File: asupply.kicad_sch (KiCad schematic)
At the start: 98 parts, among them U10 LT3081xDF, U11 LT3042xMSE, U12 LT3045xMSE, U13 LT3045xMSE, U14 LT3042xMSE, U15 LT3094xMSE, U16 LT3042xMSE, U9 LTC3261

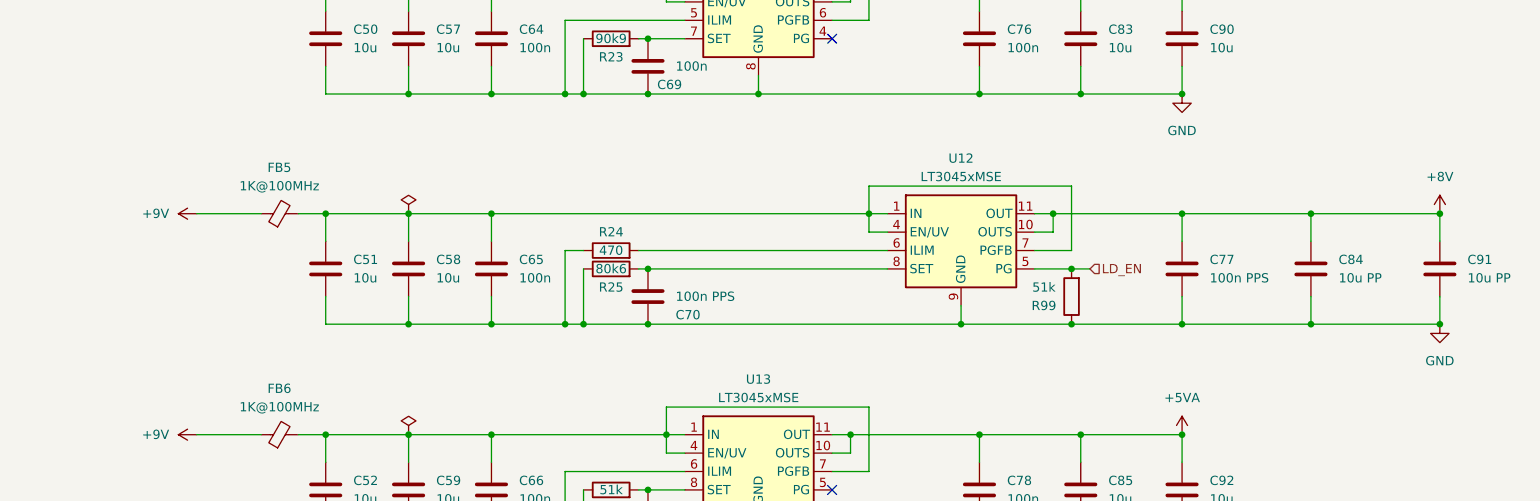
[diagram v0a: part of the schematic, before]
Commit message: sch: Fix Issue #14
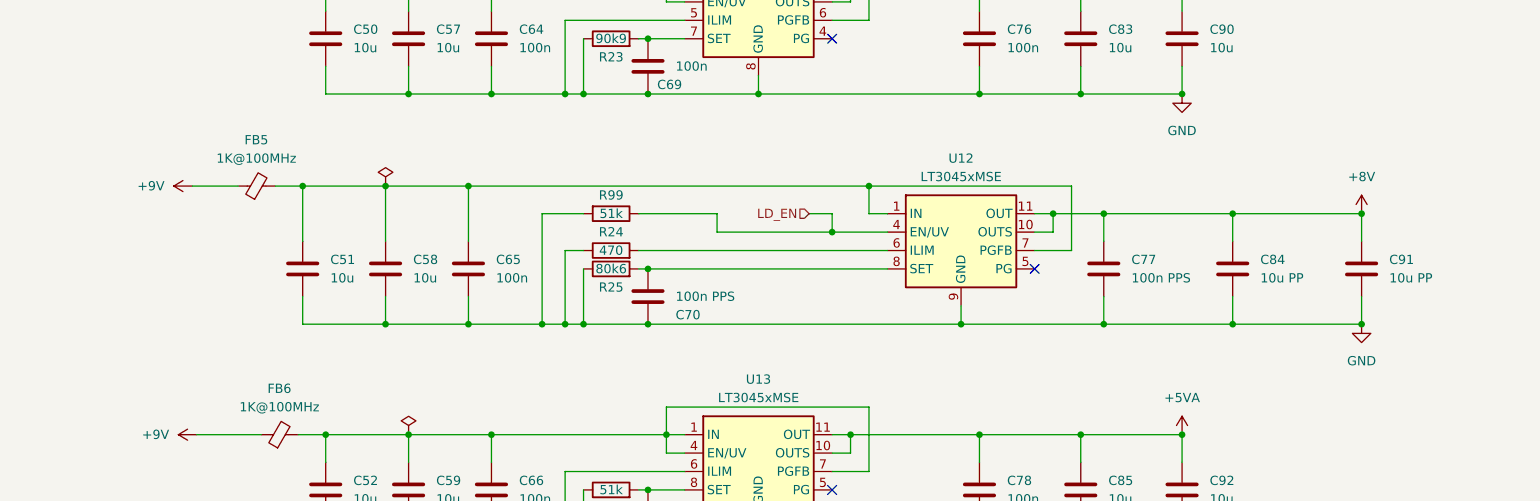
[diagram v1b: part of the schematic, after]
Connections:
- net GND: now also R99.2; no longer R99.1
- net LD_EN: now also R99.1, U12.4 (EN/UV); no longer R99.2, U12.5 (PG)
- net at C51.1, C58.1, C65.1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: no longer U12.4 (EN/UV)
- no-connect marks 7 -> 8
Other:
- moved on the sheet: C51, C58, C65, C77, C84, C91, FB5
